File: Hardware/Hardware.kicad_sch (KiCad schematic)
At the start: 47 parts, among them J1 USB_C_Receptacle_USB2.0_16P, J2 Conn_01x02_Socket, J3 Conn_01x04_Pin, Q1 AO3400A, Q2 AO3401A, SW2 ON, U1 CH32V203CxTx, U2 AMS1117-3.3, U3 TP4056-42-ESOP8

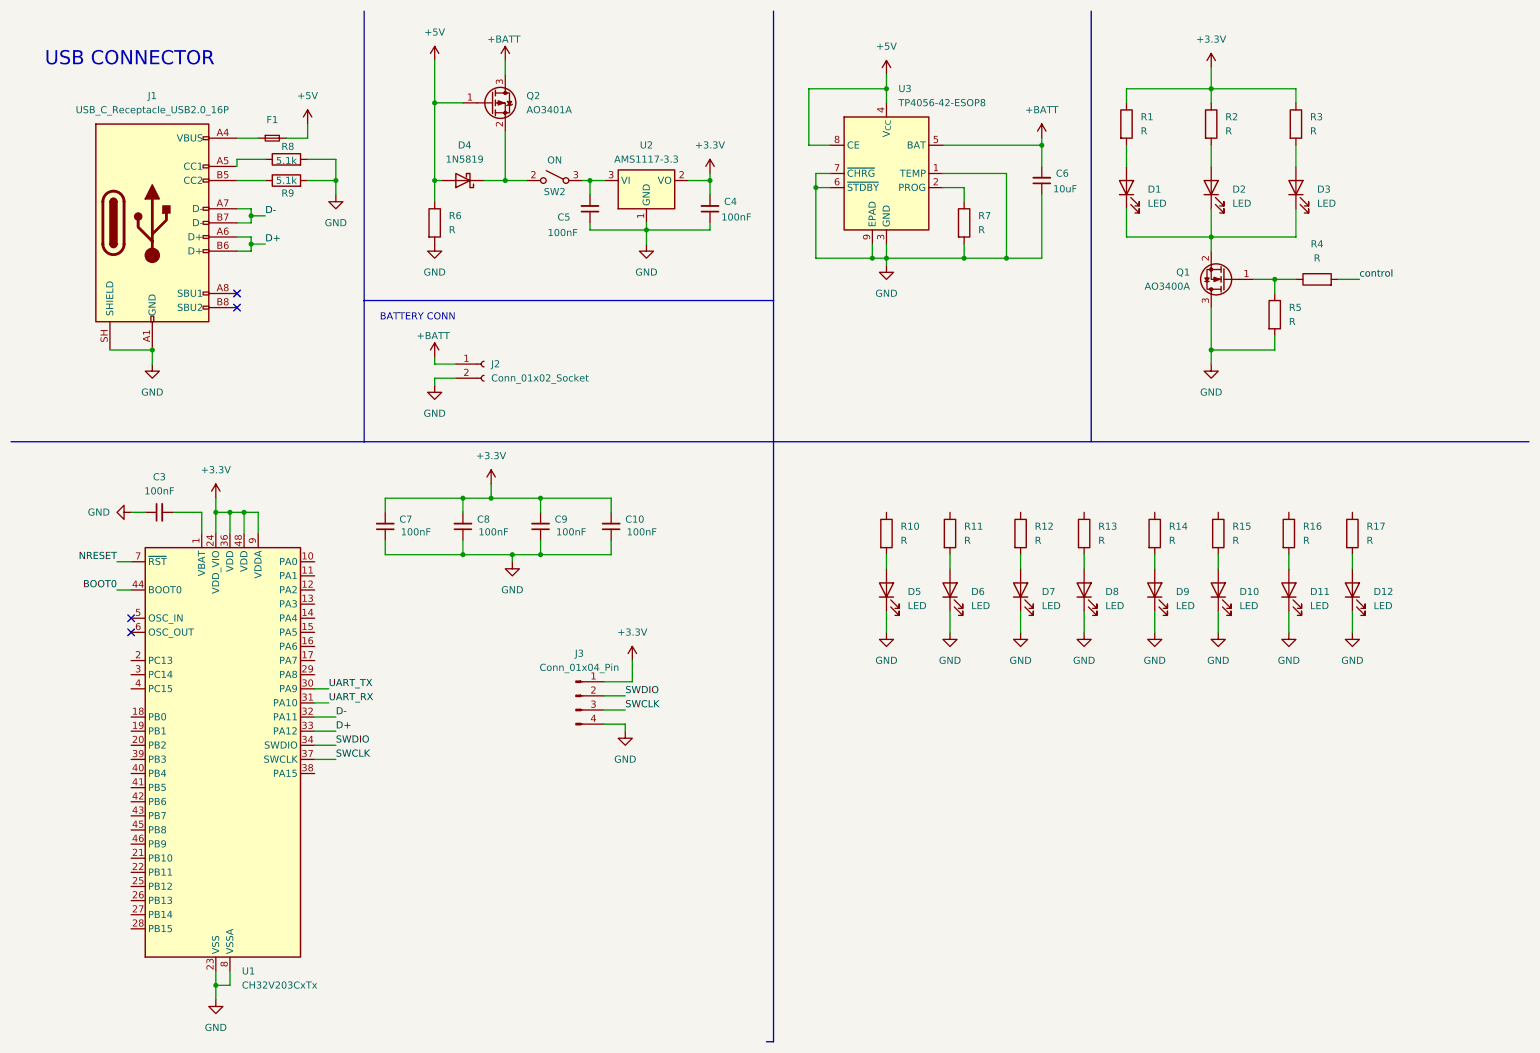
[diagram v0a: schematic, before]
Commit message: feat: add components on pcb
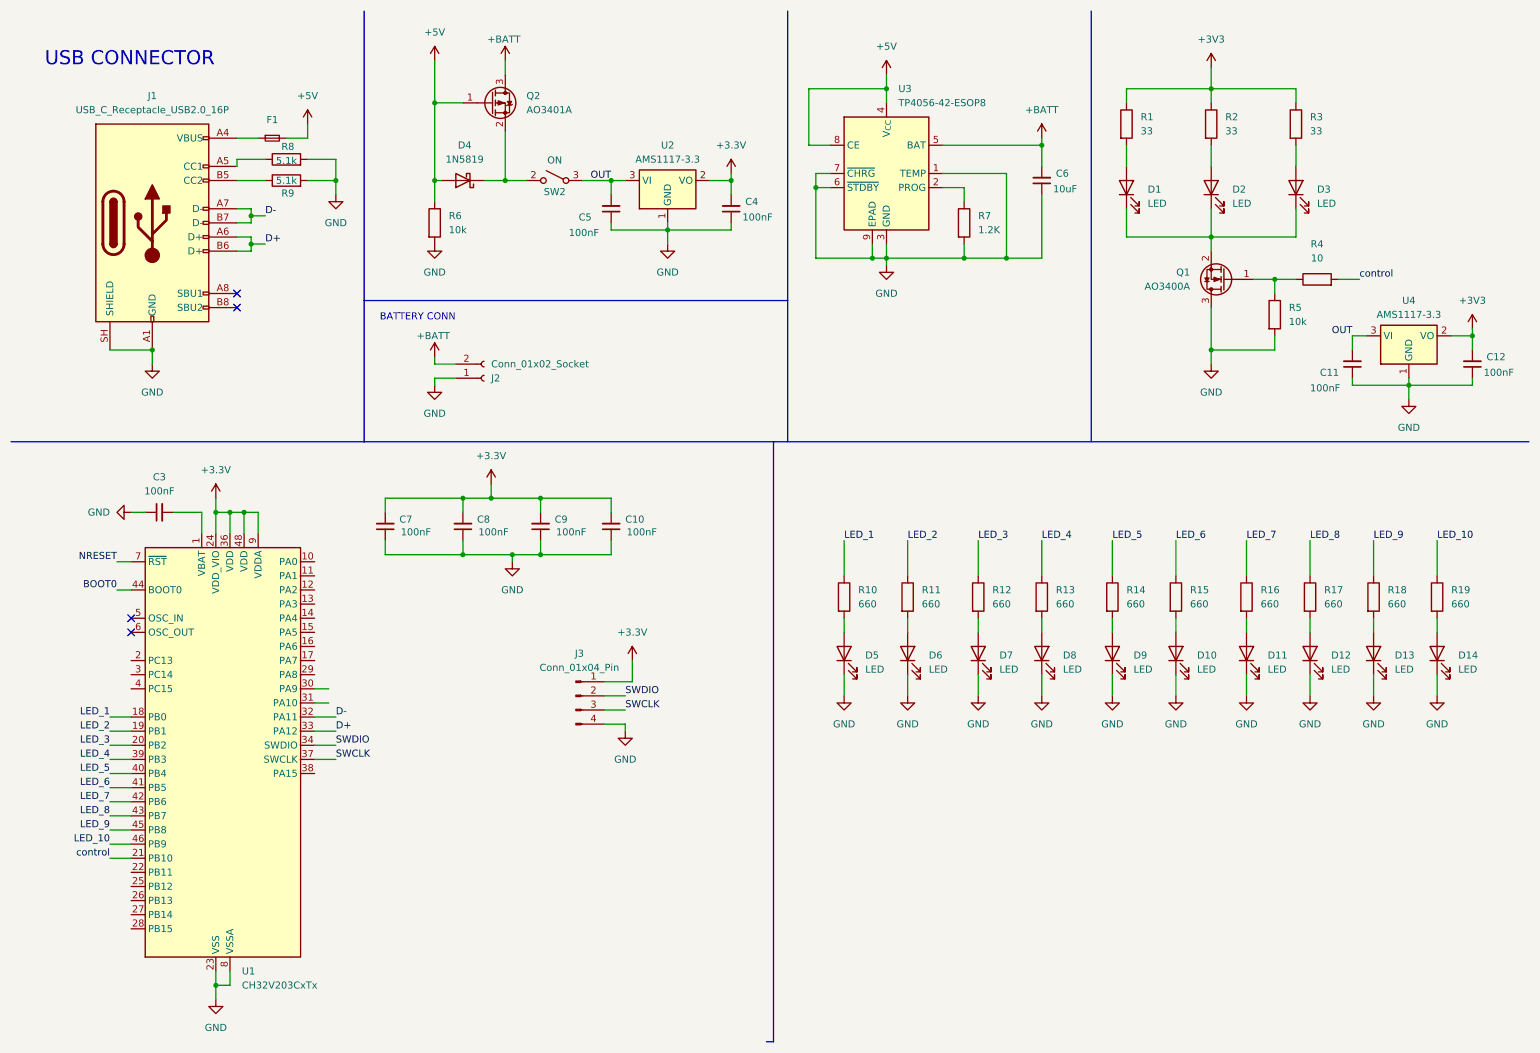
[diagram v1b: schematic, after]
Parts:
- added C11, C12: 100nF, Capacitor_SMD:C_0805_2012Metric, symbol Device:C_Small
- added D13, D14: LED, LED_SMD:LED_0603_1608Metric, symbol Device:LED
- added R18, R19: 660, Resistor_SMD:R_0805_2012Metric, symbol Device:R
- added U4: AMS1117-3.3, Package_TO_SOT_SMD:SOT-223-3_TabPin2, symbol Regulator_Linear:AMS1117-3.3
- D1, D2: footprint (none) -> Connector_PinHeader_1.27mm:PinHeader_1x02_P1.27mm_Vertical
- D10, D11, D12, D5, D6, D7, D8, D9: footprint LED_SMD:LED_Cree-XHP50_3V_HighDensity -> LED_SMD:LED_0603_1608Metric
- D4: footprint Diode_THT:D_DO-41_SOD81_P10.16mm_Horizontal -> Diode_SMD:D_SOD-323
- F1: footprint Package_SO:SOIC-8-1EP_3.9x4.9mm_P1.27mm_EP2.41x3.3mm_ThermalVias -> Fuse:Fuse_0603_1608Metric
- J1: footprint (none) -> Connector_USB:USB_C_Receptacle_Palconn_UTC16-G
- J2: footprint Package_DFN_QFN:QFN-40-1EP_6x6mm_P0.5mm_EP4.6x4.6mm -> Connector_JST:JST_PH_S2B-PH-SM4-TB_1x02-1MP_P2.00mm_Horizontal
- J3: footprint (none) -> Connector_PinHeader_2.54mm:PinHeader_1x04_P2.54mm_Vertical
- R1, R2, R3: value R -> 33; footprint (none) -> Resistor_SMD:R_0805_2012Metric
- R10, R11, R12, R13, R14, R15, R16, R17: value R -> 660; footprint (none) -> Resistor_SMD:R_0805_2012Metric
- R4: value R -> 10; footprint (none) -> Resistor_SMD:R_0805_2012Metric
- R5: value R -> 10k; footprint (none) -> Resistor_SMD:R_0805_2012Metric
- R6: value R -> 10k; footprint Package_TO_SOT_SMD:SOT-223-3_TabPin2 -> Resistor_SMD:R_0805_2012Metric
- R7: value R -> 1.2K; footprint (none) -> Resistor_SMD:R_0805_2012Metric
- SW2: footprint Footprints:MSK12C02 -> Button_Switch_SMD:SW_SPDT_Shouhan_MSK12C02
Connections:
- net +3.3V: no longer R1.1, R2.1, R3.1
- net +BATT: now also J2.2 (Pin_2); no longer J2.1 (Pin_1)
- net GND: now also J2.1 (Pin_1), C11.1, C12.1, D13.1 (K), D14.1 (K), U4.1 (GND); no longer J2.2 (Pin_2)
- net control: now also U1.21 (PB10)
- net OUT: now reaches C5.2, SW2.3 (A), U2.3 (VI)
- net OUT: now also C11.2, U4.3 (VI)
- net LED_1: now reaches R10.1
- net LED_1: now also U1.18 (PB0)
- net LED_2: now reaches R11.1
- net LED_2: now also U1.19 (PB1)
- net LED_3: now reaches R12.1
- net LED_3: now also U1.20 (PB2)
- net LED_6: now reaches R15.1
- net LED_6: now also U1.41 (PB5)
- net LED_8: now reaches R17.1
- net LED_8: now also U1.43 (PB7)
- net LED_5: now reaches R14.1
- net LED_5: now also U1.40 (PB4)
- net LED_4: now reaches U1.39 (PB3)
- net LED_4: now also R13.1
- net LED_7: now reaches U1.42 (PB6)
- net LED_7: now also R16.1
- net LED_9: now reaches U1.45 (PB8)
- net LED_9: now also R18.1
- net LED_10: now reaches U1.46 (PB9)
- net LED_10: now also R19.1
- net UART_RX: no longer names the net of U1.31 (PA10)
- net UART_TX: no longer names the net of U1.30 (PA9)
- new net: D13.2 (A), R18.2
- new net: D14.2 (A), R19.2
- new net +3V3: C12.2, R1.1, R2.1, R3.1, U4.2 (VO)
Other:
- moved on the sheet: C4, C5, D10, D11, D12, D5, D6, D7, D8, D9, R10, R11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
